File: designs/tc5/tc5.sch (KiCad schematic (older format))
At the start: 10 parts, among them J1001 SSM-104-L-SV, U1001 MCP6001-OT

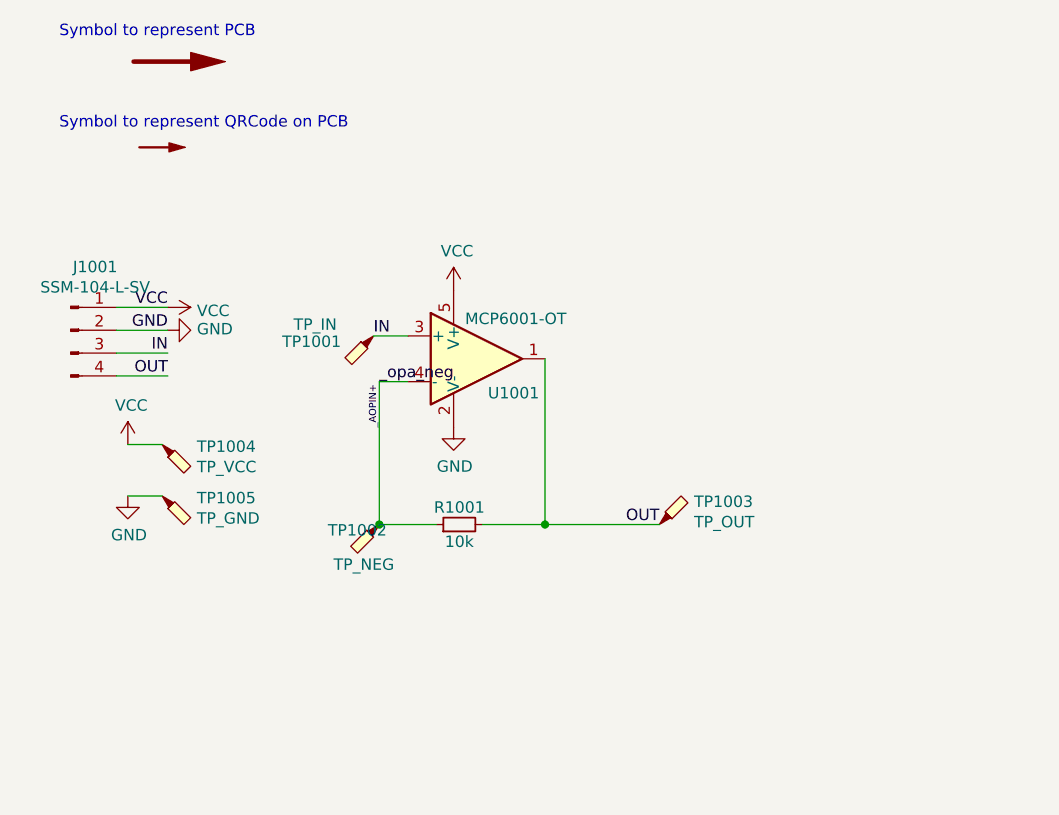
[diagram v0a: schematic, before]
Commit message: Addec TC2030 for OAR
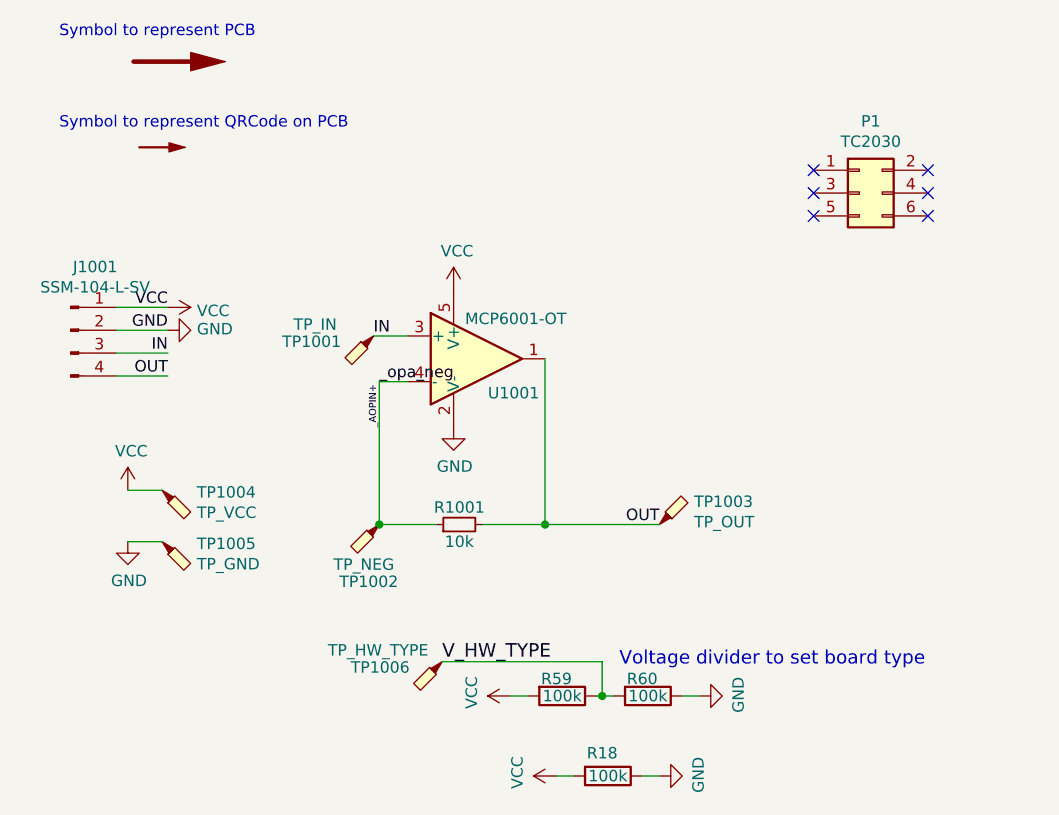
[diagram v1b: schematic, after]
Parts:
- added P1: TC2030, tc5:TC2030-MCP-FP, symbol Connector_Generic:Conn_02x03_Odd_Even
- added R18, R59, R60: 100k, Resistor_SMD:R_0603_1608Metric, symbol Device:R
- added TP1006: TP_HW_TYPE, TestPoint:TestPoint_Pad_D1.5mm, symbol tc5-rescue:TestPoint_Probe-Connector
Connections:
- net GND: now also R18.1, R60.1
- net VCC: now also R18.2, R59.2
- new net V_HW_TYPE: R59.1, R60.2, TP1006.1
- no-connect marks 0 -> 6
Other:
- note added: "Voltage divider to set board type"
- moved on the sheet: TP1004, TP1005
